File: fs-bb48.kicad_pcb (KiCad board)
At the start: 2 copper layers, 35 x 12.1 mm, 19 parts, among them P1 USB, P2 SWD, P3 PWR, P4 EXT, T1 TOUCH_PAD, U1 MKL27Z256VFM4, U2 NUP2114

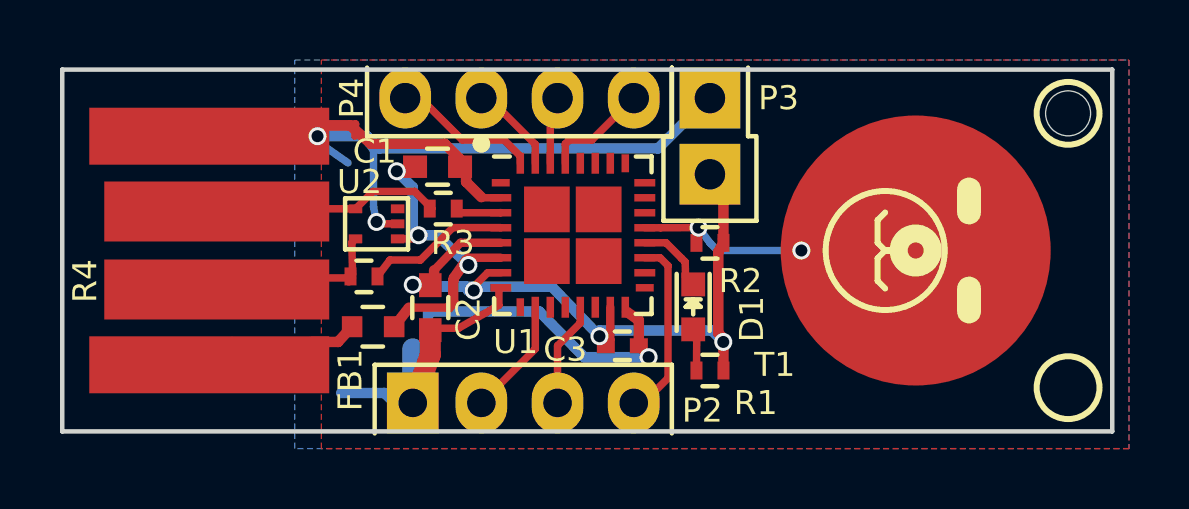
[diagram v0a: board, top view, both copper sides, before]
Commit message: fix GND line
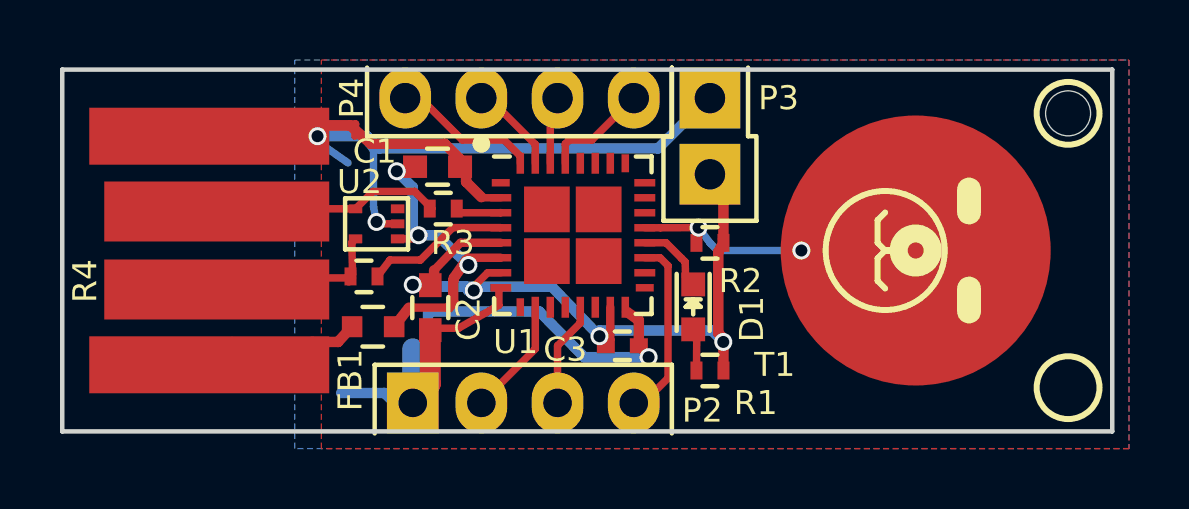
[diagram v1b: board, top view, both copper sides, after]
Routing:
- net GND: track 61.5 -> 60.8 mm
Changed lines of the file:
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@@
   (segment (start 138.8244 109.5248) (end 138.7602 109.589) (width 0.25) (layer F.Cu) (net 1) (status 30))
   (segment (start 138.5944 109.4232) (end 138.7602 109.589) (width 0.35) (layer F.Cu) (net 1) (status 30))
-  (segment (start 138.7602 109.589) (end 138.7602 110.4138) (width 0.7) (layer F.Cu) (net 1) (status 10))
-  (segment (start 138.7602 110.4138) (end 138.176 112.014) (width 0.7) (layer F.Cu) (net 1))
+  (segment (start 138.7602 109.589) (end 138.7602 111.379) (width 0.7) (layer F.Cu) (net 1) (status 10))
+  (segment (start 138.7602 111.379) (end 138.176 112.014) (width 0.7) (layer F.Cu) (net 1))
   (segment (start 145.711 110.109) (end 145.711 110.1637) (width 0.25) (layer F.Cu) (net 1))
   (segment (start 145.711 110.1637) (end 146.0373 110.49) (width 0.25) (layer F.Cu) (net 1))
@@
   (segment (start 139.7635 104.152) (end 139.7515 104.14) (width 0.25) (layer F.Cu) (net 1) (status 30))
   (segment (start 138.7602 109.589) (end 138.7094 109.6264) (width 0.25) (layer F.Cu) (net 1) (status 30))
-  (segment (start 138.557 110.617) (end 138.176 112.014) (width 0.25) (layer F.Cu) (net 1))
+  (segment (start 138.557 111.5822) (end 138.176 112.014) (width 0.25) (layer F.Cu) (net 1))
   (segment (start 145.2984 108.9787) (end 145.3134 108.9787) (width 0.25) (layer F.Cu) (net 1))
   (segment (start 145.3134 108.9787) (end 145.711 109.262) (width 0.35) (layer F.Cu) (net 1))
